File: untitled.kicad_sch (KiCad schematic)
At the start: 42 parts, among them SW1 Switch, SW10 Switch, SW11 Switch, SW12 Switch, SW13 Switch, SW14 Switch, SW15 Switch, SW16 Switch, SW17 Switch, SW18 Switch, SW19 Switch, SW2 Switch, SW20 Switch, SW21 RotaryEncoder_Switch, SW3 Switch, SW4 Switch, SW5 Switch, SW6 Switch, SW7 Switch, SW8 Switch, SW9 Switch

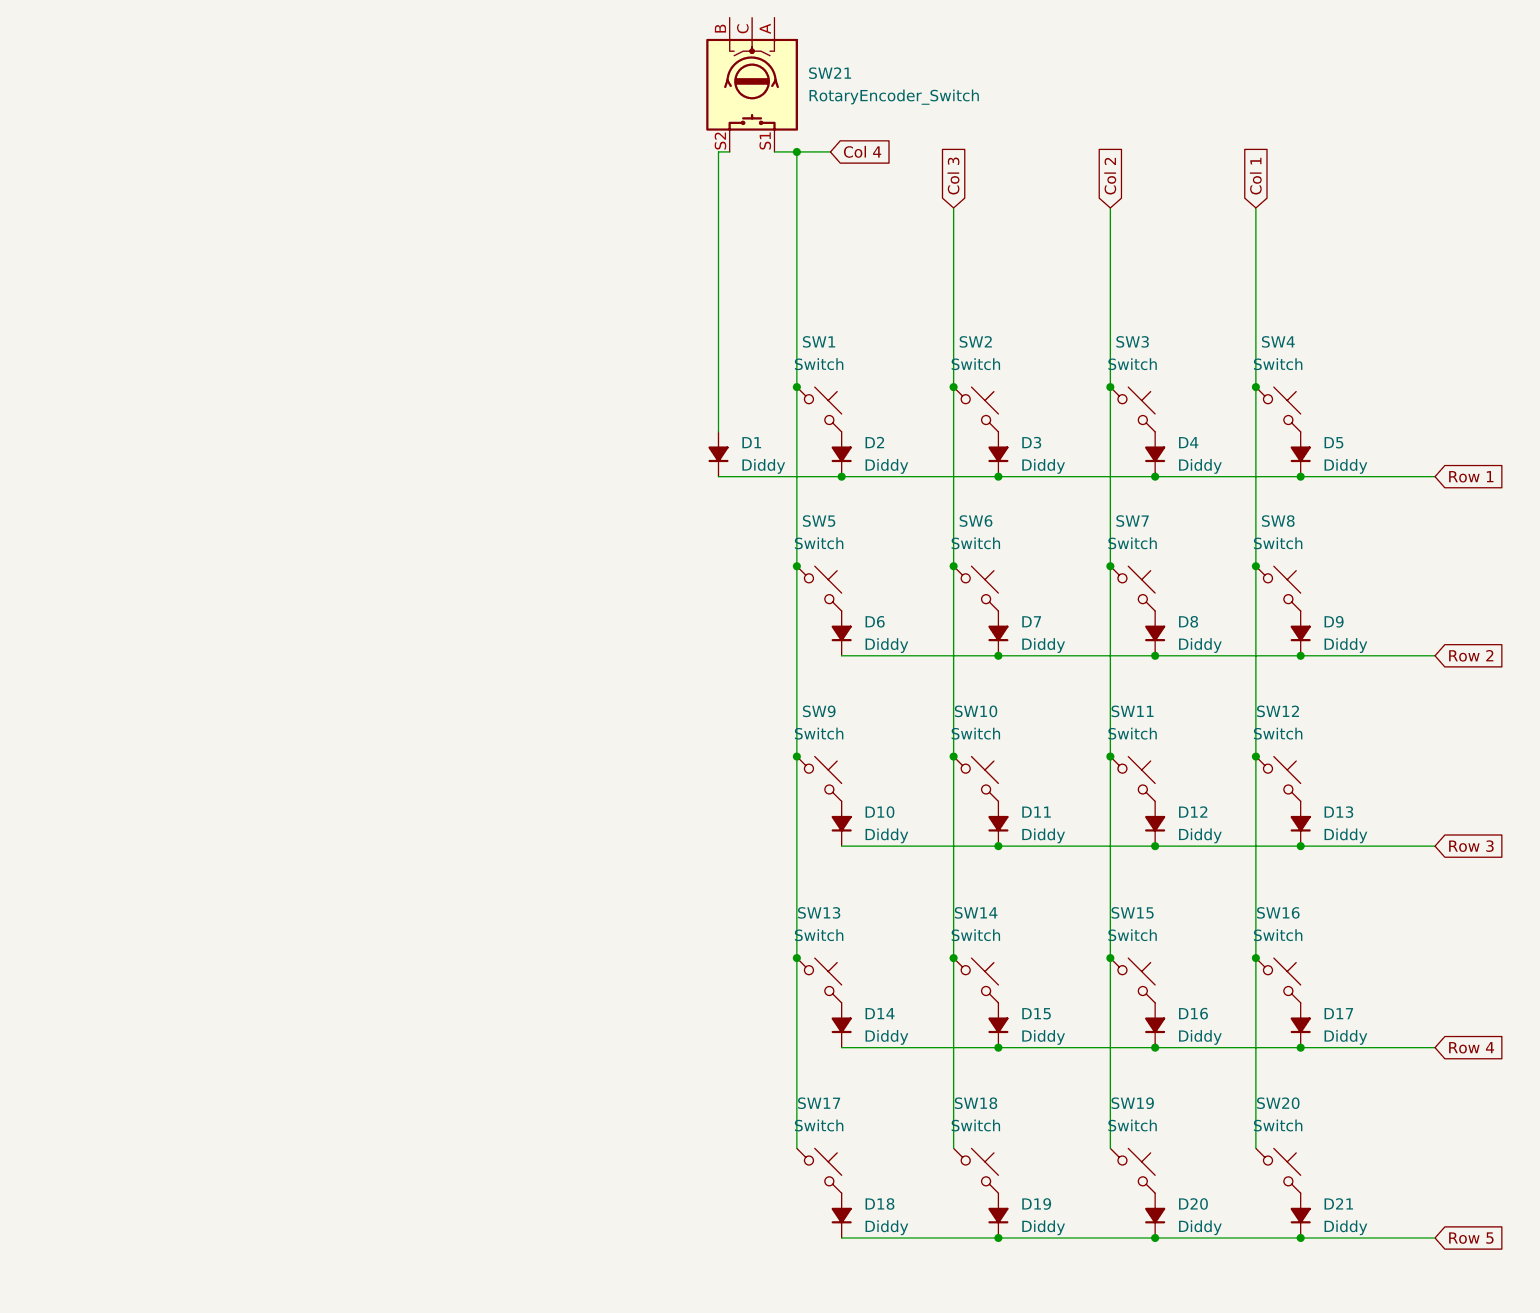
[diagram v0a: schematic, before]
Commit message: pcb
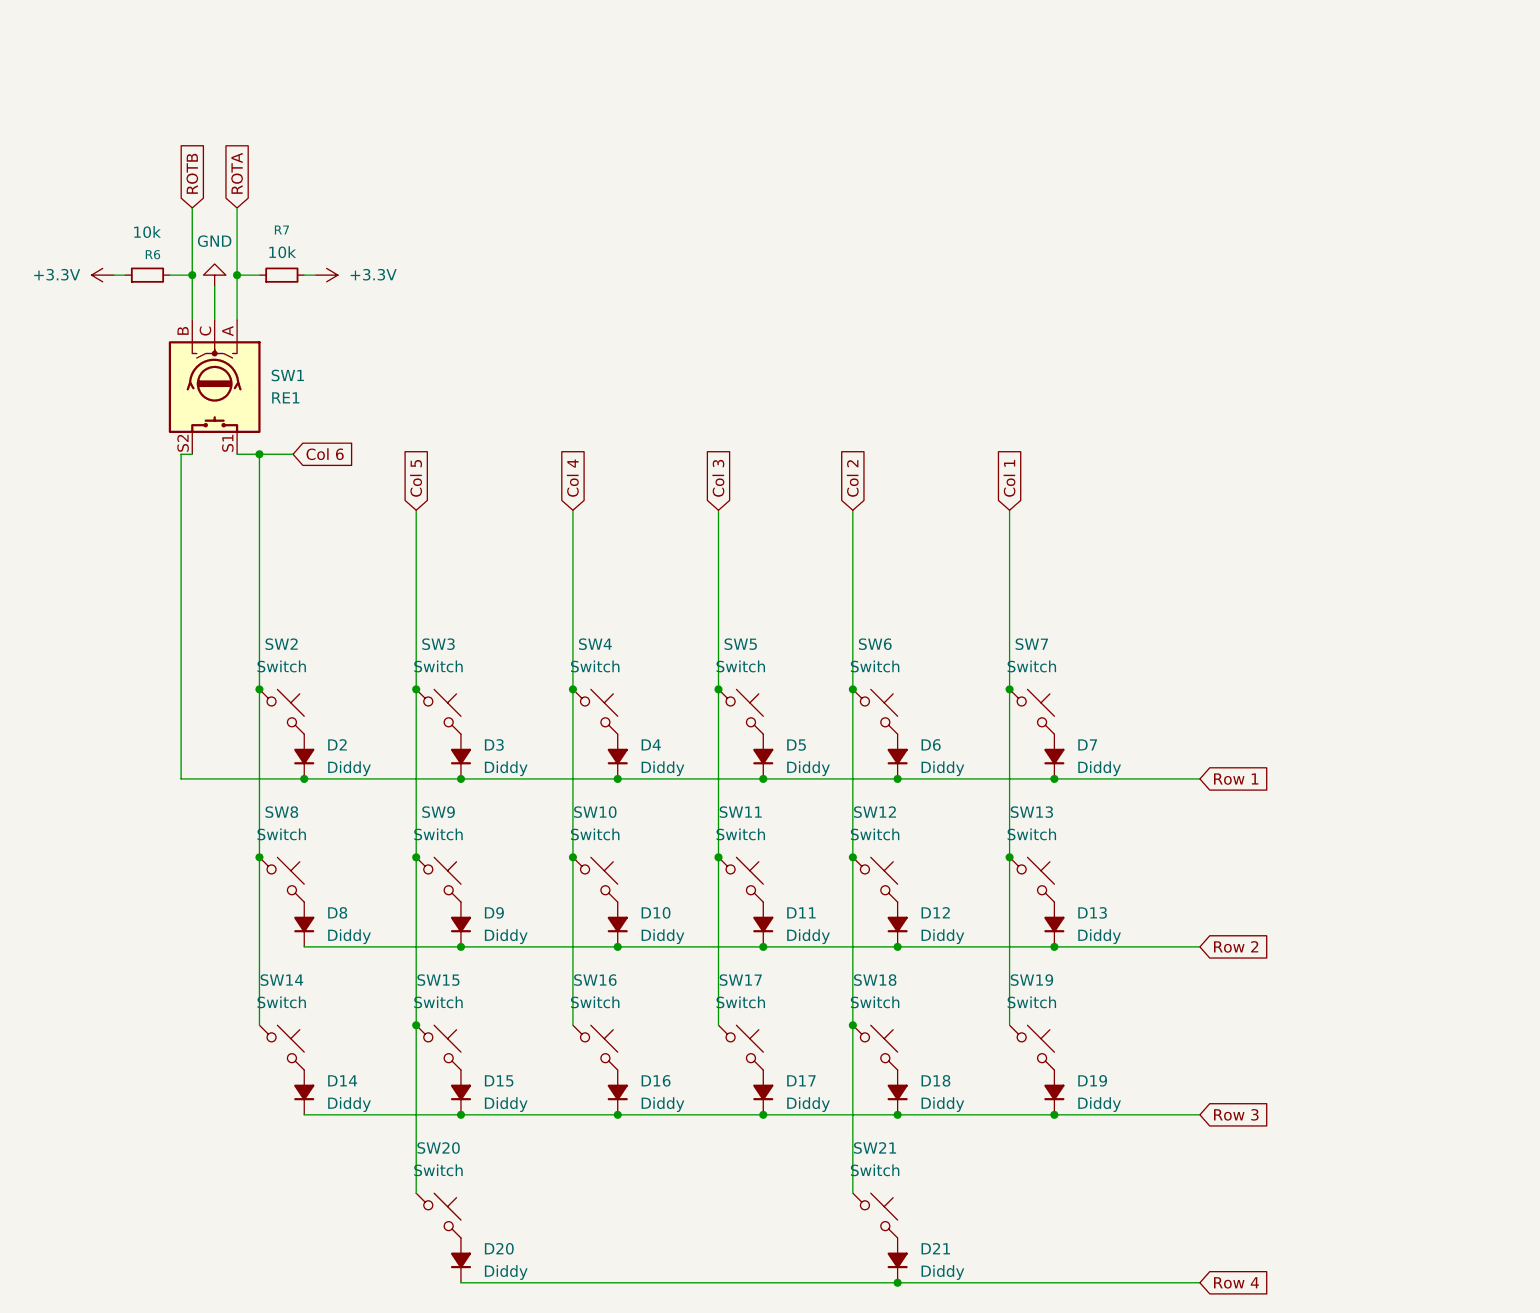
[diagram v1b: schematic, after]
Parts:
- removed D1: Diddy, symbol Device:D_Small_Filled
- added R6, R7: 10k, Resistor_SMD:R_0805_2012Metric, symbol Device:R_Small
- D10, D11, D12, D13, D14, D15, D16, D17, D18, D19, D2, D20, D21, D3, D4, D5, D6, D7, D8, D9: footprint (none) -> Diode_SMD:D_SOD-123
- SW1: renamed from SW21; value RotaryEncoder_Switch -> RE1; footprint (none) -> PCM_marbastlib-various:ROT_Alps_EC11E-Switch
- SW10: renamed from SW9; footprint (none) -> PCM_marbastlib-mx:SW_MX_HS_CPG151101S11_1u
- SW11: renamed from SW10; footprint (none) -> PCM_marbastlib-mx:SW_MX_HS_CPG151101S11_1u
- SW12: renamed from SW11; footprint (none) -> PCM_marbastlib-mx:SW_MX_HS_CPG151101S11_1u
- SW13: renamed from SW12; footprint (none) -> PCM_marbastlib-mx:SW_MX_HS_CPG151101S11_1u
- SW14: renamed from SW13; footprint (none) -> PCM_marbastlib-mx:SW_MX_HS_CPG151101S11_1u
- SW15: renamed from SW14; footprint (none) -> PCM_marbastlib-mx:SW_MX_HS_CPG151101S11_1u
- SW16: renamed from SW15; footprint (none) -> PCM_marbastlib-mx:SW_MX_HS_CPG151101S11_1u
- SW17: renamed from SW16; footprint (none) -> PCM_marbastlib-mx:SW_MX_HS_CPG151101S11_1u
- SW18: renamed from SW17; footprint (none) -> PCM_marbastlib-mx:SW_MX_HS_CPG151101S11_1u
- SW19: renamed from SW18; footprint (none) -> PCM_marbastlib-mx:SW_MX_HS_CPG151101S11_1u
- SW2: renamed from SW1; footprint (none) -> PCM_marbastlib-mx:SW_MX_HS_CPG151101S11_1u
- SW20: renamed from SW19; footprint (none) -> PCM_marbastlib-mx:SW_MX_HS_CPG151101S11_1u
- SW21: renamed from SW20; footprint (none) -> PCM_marbastlib-mx:SW_MX_HS_CPG151101S11_1u
- SW3: renamed from SW2; footprint (none) -> PCM_marbastlib-mx:SW_MX_HS_CPG151101S11_1u
- SW4: renamed from SW3; footprint (none) -> PCM_marbastlib-mx:SW_MX_HS_CPG151101S11_1u
- SW5: renamed from SW4; footprint (none) -> PCM_marbastlib-mx:SW_MX_HS_CPG151101S11_1u
- SW6: renamed from SW5; footprint (none) -> PCM_marbastlib-mx:SW_MX_HS_CPG151101S11_1u
- SW7: renamed from SW6; footprint (none) -> PCM_marbastlib-mx:SW_MX_HS_CPG151101S11_1u
- SW8: renamed from SW7; footprint (none) -> PCM_marbastlib-mx:SW_MX_HS_CPG151101S11_1u
- SW9: renamed from SW8; footprint (none) -> PCM_marbastlib-mx:SW_MX_HS_CPG151101S11_1u
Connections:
- net Col 1: now also SW19.1, SW7.1; no longer SW17.1, SW21.1, SW5.1, SW9.1
- net Col 2: now also SW18.1, SW21.1, SW6.1; no longer SW16.1, SW20.1, SW4.1, SW8.1
- net Col 3: now also SW17.1, SW5.1; no longer SW15.1, SW19.1, SW3.1, SW7.1
- net Col 4: now also SW16.1, SW4.1; no longer SW1.S1, SW14.1, SW18.1, SW2.1, SW6.1
- net Row 1: now also D6.1 (K), D7.1 (K), SW1.S2
- net Row 2: now also D10.1 (K), D11.1 (K), D12.1 (K), D13.1 (K); no longer D6.1 (K), D7.1 (K)
- net Row 3: now also D14.1 (K), D15.1 (K), D16.1 (K), D17.1 (K), D18.1 (K), D19.1 (K); no longer D10.1 (K), D11.1 (K), D12.1 (K), D13.1 (K)
- net Row 4: now also D20.1 (K), D21.1 (K); no longer D14.1 (K), D15.1 (K), D16.1 (K), D17.1 (K)
- net ROTA: now reaches SW1.A
- net ROTA: now also R7.1
- net ROTB: now reaches SW1.B
- net ROTB: now also R6.2
- net GND: now reaches SW1.C
- removed net Row 5: D18.1 (K), D19.1 (K), D20.1 (K), D21.1 (K)
- new net +3.3V: R6.1, R7.2
- new net Col 5: SW15.1, SW20.1, SW3.1, SW9.1
- new net Col 6: SW1.S1, SW14.1, SW2.1, SW8.1
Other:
- moved on the sheet: D10, D11, D12, D13, D14, D15, D16, D17, D18, D19, D2, D20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
